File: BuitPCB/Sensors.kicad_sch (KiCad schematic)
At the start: 3 parts, among them J5 LEFT VL, J7 RIGHT VL, J9 CENTER VL

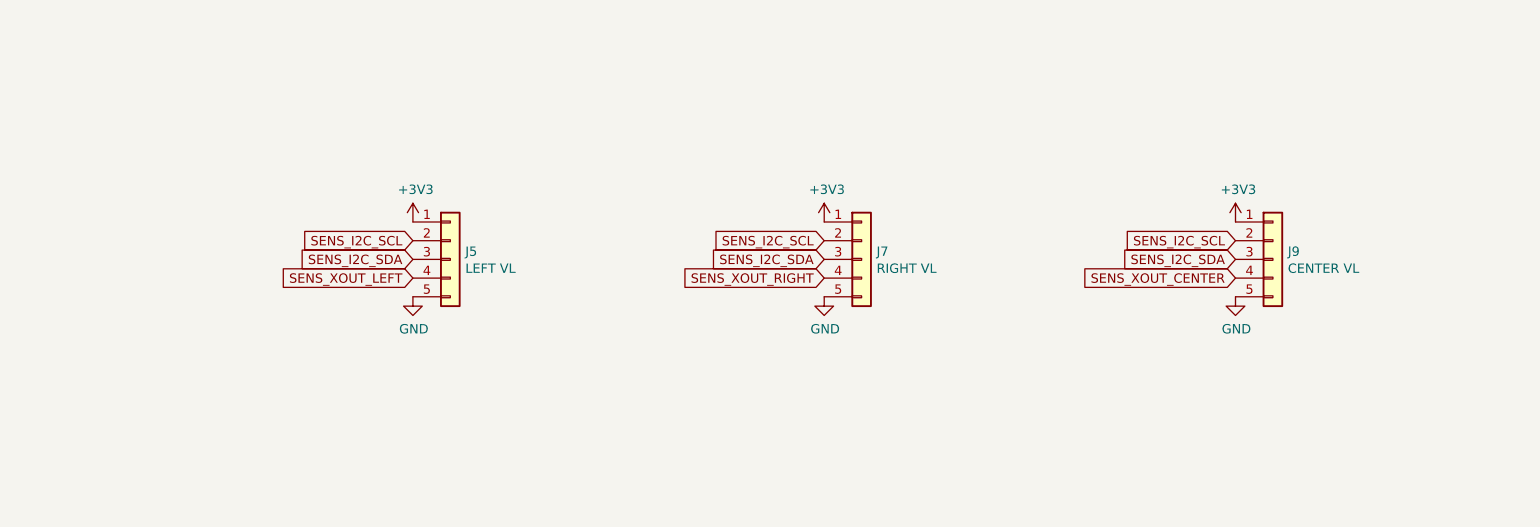
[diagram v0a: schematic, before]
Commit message: Updated almost to final 0.1 version
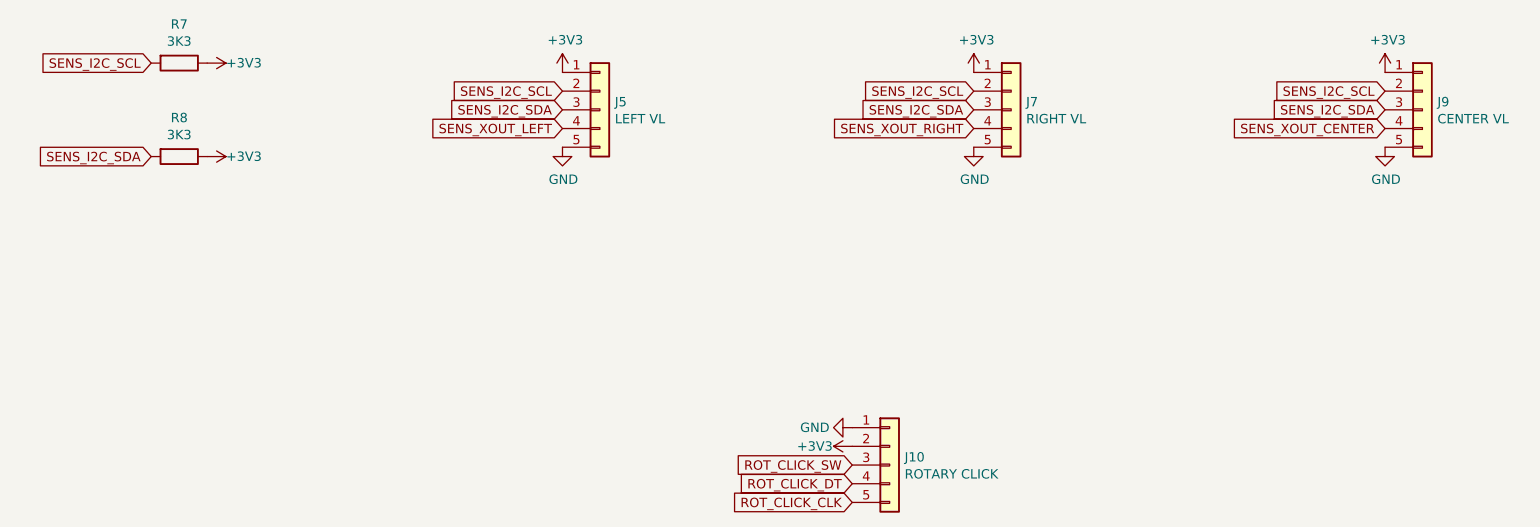
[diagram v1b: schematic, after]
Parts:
- added J10: ROTARY CLICK, Connector_JST:JST_XH_B5B-XH-A_1x05_P2.50mm_Vertical, symbol Connector_Generic:Conn_01x05
- added R7, R8: 3K3, Resistor_SMD:R_0805_2012Metric, symbol Device:R
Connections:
- net +3V3: now also J10.2 (Pin_2), R7.1, R8.1
- net GND: now also J10.1 (Pin_1)
- net SENS_I2C_SCL: now also R7.2
- net SENS_I2C_SDA: now also R8.2
- new net ROT_CLICK_CLK: J10.5 (Pin_5)
- new net ROT_CLICK_DT: J10.4 (Pin_4)
- new net ROT_CLICK_SW: J10.3 (Pin_3)
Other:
- moved on the sheet: J5, J7, J9
